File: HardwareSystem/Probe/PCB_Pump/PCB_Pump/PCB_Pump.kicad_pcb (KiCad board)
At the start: 2 copper layers, 40.9 x 43.2 mm, 15 parts, among them Q1 IRF510, U1 LM2937xT

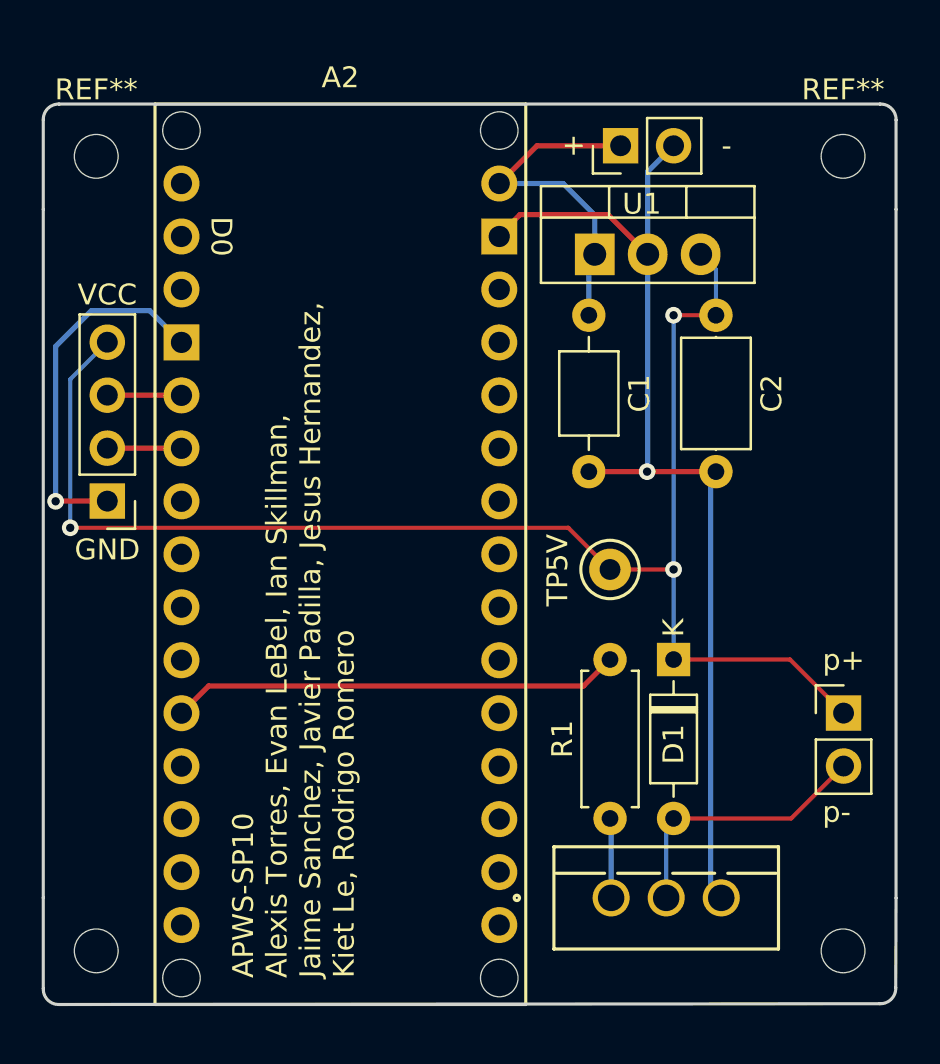
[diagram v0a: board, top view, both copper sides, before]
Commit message: pumpv2-v3
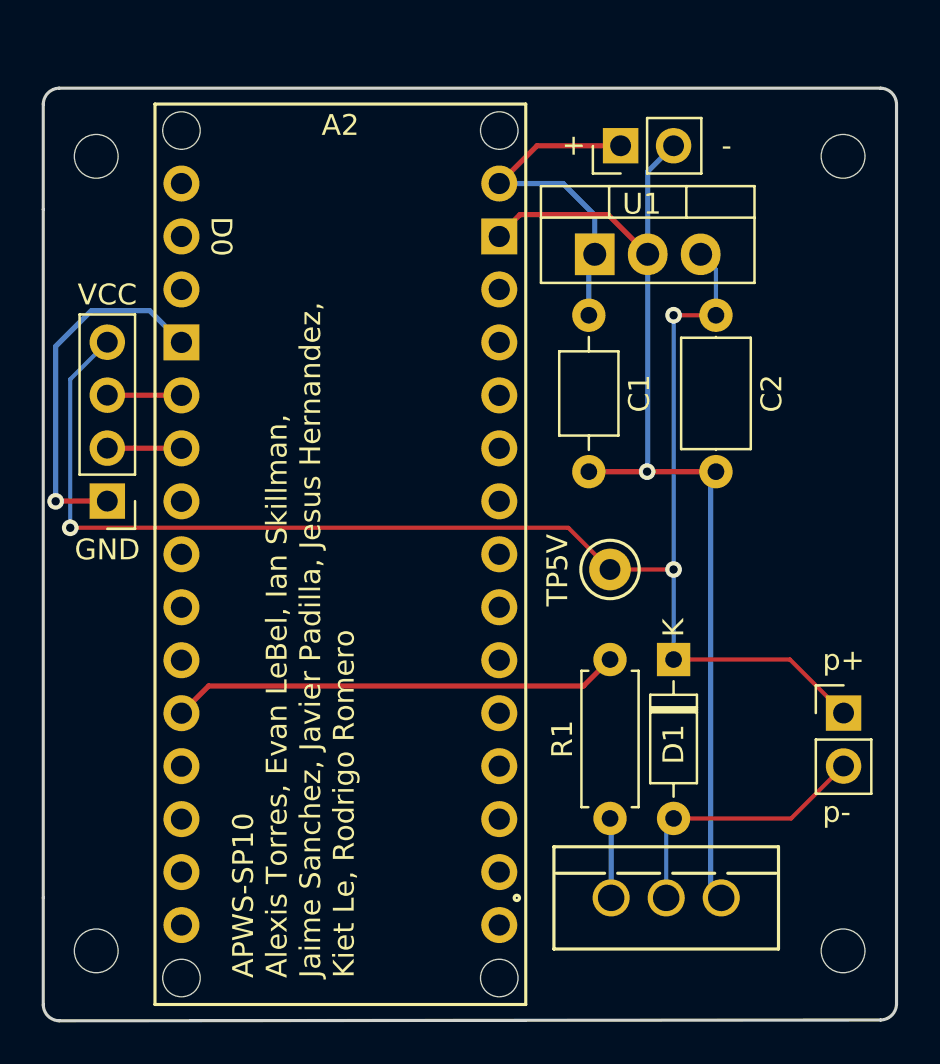
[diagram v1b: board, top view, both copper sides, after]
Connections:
- A2 pad GND2: Net-(A2-GND-PadGND1) -> GND
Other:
- board size 40.9 x 43.2 mm -> 40.9 x 44.7 mm
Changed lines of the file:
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@@
   (net 31 "unconnected-(A2-Pad5V)")
   (net 32 "9V")
-  (net 33 "Net-(A2-GND-PadGND1)")
   (footprint "Connector_PinHeader_2.54mm:PinHeader_1x02_P2.54mm_Vertical" (layer "F.Cu")
     (at 153.416 99.309)
@@
     (tags "mounting hole 2.1mm no annular")
     (attr exclude_from_pos_files exclude_from_bom)
-    (fp_text reference "REF**" (at 0 -3.2) (layer "F.SilkS")
+    (fp_text reference "REF**" (at 0 -3.2) (layer "F.SilkS") hide
         (effects (font (size 1 1) (thickness 0.15)))
     )
@@
     (tags "mounting hole 2.1mm no annular")
     (attr exclude_from_pos_files exclude_from_bom)
-    (fp_text reference "REF**" (at 0 -3.2) (layer "F.SilkS")
+    (fp_text reference "REF**" (at 0 -3.2) (layer "F.SilkS") hide
         (effects (font (size 1 1) (thickness 0.15)))
     )
@@
     (property "ki_description" "MOSFET RECOMMENDED ALT 844-IRF510PBF")
     (attr through_hole)
-    (fp_text reference "Q1" (at -0.35 0 unlocked) (layer "B.SilkS")
+    (fp_text reference "Q1" (at -0.031 1.8107 unlocked) (layer "B.SilkS")
         (effects (font (size 1 1) (thickness 0.15)) (justify mirror))
     )
@@
     (property "ki_keywords" "Arduino MPU Shield")
     (attr through_hole)
-    (fp_text reference "A2" (at 0 -44.45) (layer "F.SilkS")
+    (fp_text reference "A2" (at 0 -42.164) (layer "F.SilkS")
         (effects (font (size 1 1) (thickness 0.15)))
     )
@@
       (net 3 "GND") (pinfunction "GND") (pintype "power_in"))
     (pad "GND2" thru_hole rect (at 7.62 -36.83) (size 1.7272 1.7272) (drill 1.016) (layers "*.Cu" "*.Mask")
-      (net 33 "Net-(A2-GND-PadGND1)") (pinfunction "GND") (pintype "power_in"))
+      (net 3 "GND") (pinfunction "GND") (pintype "power_in"))
     (pad "RST" thru_hole circle (at -7.62 -34.29) (size 1.7272 1.7272) (drill 1.016) (layers "*.Cu" "*.Mask")
       (net 30 "unconnected-(A2-~{RESET}-PadRST)") (pinfunction "~{RESET}") (pintype "open_collector"))
@@
     (pad "" np_thru_hole circle (at 0 0) (size 2.1 2.1) (drill 2.1) (layers "F&B.Cu" "*.Mask"))
   )
-  (gr_arc (start 115.038999 70.866) (mid 115.255166 70.320167) (end 115.800999 70.104)
-    (stroke (width 0.15) (type default)) (layer "Edge.Cuts"))
-  (gr_line (start 155.932999 108.1713) (end 155.932999 75.1513)
-    (stroke (width 0.15) (type default)) (layer "Edge.Cuts"))
-  (gr_line (start 115.800999 70.104) (end 155.170999 70.104)
-    (stroke (width 0.15) (type default)) (layer "Edge.Cuts"))
-  (gr_line (start 115.038999 70.866) (end 115.038999 75.1513)
-    (stroke (width 0.15) (type default)) (layer "Edge.Cuts"))
-  (gr_line (start 115.038999 108.1713) (end 115.038999 112.522)
-    (stroke (width 0.15) (type default)) (layer "Edge.Cuts"))
-  (gr_line (start 155.932999 108.1713) (end 155.918167 112.484167)
+  (gr_arc (start 115.038999 70.104) (mid 115.267481 69.570482) (end 115.800999 69.342)
+    (stroke (width 0.15) (type default)) (layer "Edge.Cuts"))
+  (gr_line (start 155.956 113.265083) (end 155.956 70.104)
+    (stroke (width 0.15) (type default)) (layer "Edge.Cuts"))
+  (gr_line (start 115.800999 69.342) (end 155.194 69.342)
+    (stroke (width 0.15) (type default)) (layer "Edge.Cuts"))
+  (gr_line (start 115.038999 70.104) (end 115.038999 75.1513)
+    (stroke (width 0.15) (type default)) (layer "Edge.Cuts"))
+  (gr_arc (start 155.956 113.265083) (mid 155.727518 113.798601) (end 155.194 114.027083)
+    (stroke (width 0.15) (type default)) (layer "Edge.Cuts"))
+  (gr_arc (start 155.194 69.342) (mid 155.727518 69.570482) (end 155.956 70.104)
+    (stroke (width 0.15) (type default)) (layer "Edge.Cuts"))
+  (gr_line (start 115.038999 108.1713) (end 115.038999 113.302916)
     (stroke (width 0.15) (type default)) (layer "Edge.Cuts"))
   (gr_line (start 115.038999 75.1513) (end 115.038999 108.1713)
     (stroke (width 0.15) (type default)) (layer "Edge.Cuts"))
-  (gr_arc (start 115.800999 113.284) (mid 115.255166 113.067833) (end 115.038999 112.522)
-    (stroke (width 0.15) (type default)) (layer "Edge.Cuts"))
-  (gr_line (start 115.800999 113.284) (end 155.156167 113.246167)
-    (stroke (width 0.15) (type default)) (layer "Edge.Cuts"))
-  (gr_arc (start 155.170999 70.104) (mid 155.716832 70.320167) (end 155.932999 70.866)
-    (stroke (width 0.15) (type default)) (layer "Edge.Cuts"))
-  (gr_line (start 155.932999 70.866) (end 155.932999 75.1513)
-    (stroke (width 0.15) (type default)) (layer "Edge.Cuts"))
-  (gr_arc (start 155.918167 112.484167) (mid 155.702 113.03) (end 155.156167 113.246167)
+  (gr_line (start 115.800999 114.064916) (end 155.194 114.027083)
+    (stroke (width 0.15) (type default)) (layer "Edge.Cuts"))
+  (gr_arc (start 115.800999 114.064916) (mid 115.267481 113.836434) (end 115.038999 113.302916)
     (stroke (width 0.15) (type default)) (layer "Edge.Cuts"))
   (gr_text "VCC" (at 118.11 79.248) (layer "F.SilkS")
